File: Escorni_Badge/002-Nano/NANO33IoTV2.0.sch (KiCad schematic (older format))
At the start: 10 parts, among them J1 Arduino-NANO-33

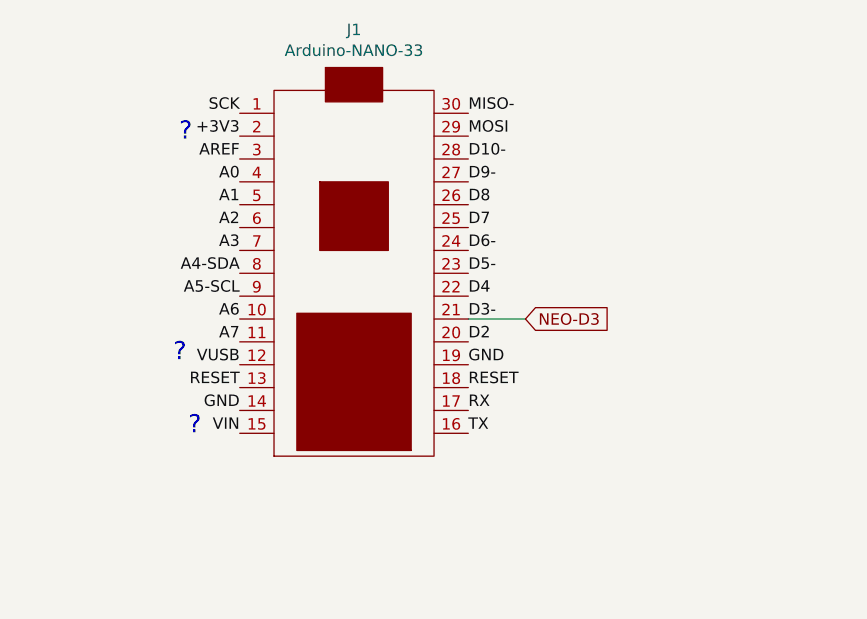
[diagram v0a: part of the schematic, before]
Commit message: Add some minors changes
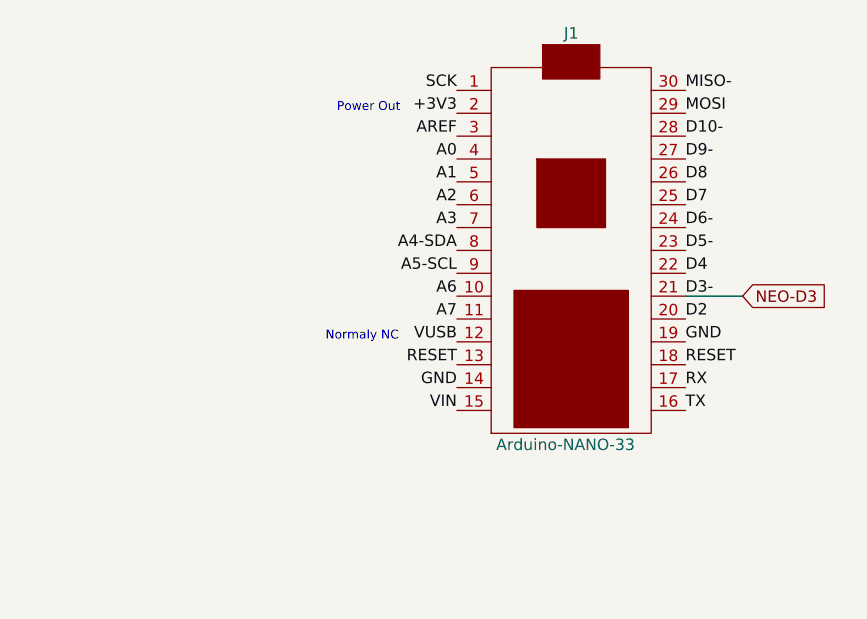
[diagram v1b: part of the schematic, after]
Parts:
- C1: footprint 002:C_1206_HandSoldering -> Capacitor_SMD:C_0805_2012Metric_Pad1.15x1.40mm_HandSolder
- J1: footprint Arduino:NANO_33_Socket_Castell -> Arduino:NANO_33_Single_Socket
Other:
- note added: "Normaly NC"
- note added: "Power Out"
- note removed: "?"
- moved on the sheet: J1
